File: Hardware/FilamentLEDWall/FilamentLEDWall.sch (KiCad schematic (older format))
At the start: 24 parts, among them J1 TopLeftConnector, J2 BottomLeftConnector, J3 BottomRightConnector, J4 TopRightConnector, U3 JXI5020GF

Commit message: Updated LED Board to v0.2
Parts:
- J1, J2, J3, J4: footprint Connector_PinHeader_2.54mm:PinHeader_2x04_P2.54mm_Vertical_SMD -> Connector_PinSocket_2.54mm:PinSocket_2x04_P2.54mm_Vertical_SMD
- U3: footprint Silicon-Standard:SSOP24 -> Sensor_Current:Allegro_QSOP-24_3.9x8.7mm_P0.635mm
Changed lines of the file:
@@
 F 0 "U3" H 8175 3515 50  0000 C CNN
 F 1 "JXI5020GF" H 8175 3424 50  0000 C CNN
-F 2 "Silicon-Standard:SSOP24" H 8500 3400 50  0001 C CNN
+F 2 "Sensor_Current:Allegro_QSOP-24_3.9x8.7mm_P0.635mm" H 8500 3400 50  0001 C CNN
 F 3 "" H 8500 3400 50  0001 C CNN
 	1    8200 2500
@@
 F 0 "J1" H 2900 6167 50  0000 C CNN
 F 1 "TopLeftConnector" H 2900 6076 50  0000 C CNN
-F 2 "Connector_PinHeader_2.54mm:PinHeader_2x04_P2.54mm_Vertical_SMD" H 2850 5850 50  0001 C CNN
+F 2 "Connector_PinSocket_2.54mm:PinSocket_2x04_P2.54mm_Vertical_SMD" H 2850 5850 50  0001 C CNN
 F 3 "~" H 2850 5850 50  0001 C CNN
 	1    2850 5850
@@
 F 0 "J2" H 2900 7167 50  0000 C CNN
 F 1 "BottomLeftConnector" H 2900 7076 50  0000 C CNN
-F 2 "Connector_PinHeader_2.54mm:PinHeader_2x04_P2.54mm_Vertical_SMD" H 2850 6850 50  0001 C CNN
+F 2 "Connector_PinSocket_2.54mm:PinSocket_2x04_P2.54mm_Vertical_SMD" H 2850 6850 50  0001 C CNN
 F 3 "~" H 2850 6850 50  0001 C CNN
 	1    2850 6850
@@
 F 0 "J4" H 4200 6167 50  0000 C CNN
 F 1 "TopRightConnector" H 4200 6076 50  0000 C CNN
-F 2 "Connector_PinHeader_2.54mm:PinHeader_2x04_P2.54mm_Vertical_SMD" H 4150 5850 50  0001 C CNN
+F 2 "Connector_PinSocket_2.54mm:PinSocket_2x04_P2.54mm_Vertical_SMD" H 4150 5850 50  0001 C CNN
 F 3 "~" H 4150 5850 50  0001 C CNN
 	1    4150 5850
@@
 F 0 "J3" H 4200 7167 50  0000 C CNN
 F 1 "BottomRightConnector" H 4200 7076 50  0000 C CNN
-F 2 "Connector_PinHeader_2.54mm:PinHeader_2x04_P2.54mm_Vertical_SMD" H 4150 6850 50  0001 C CNN
+F 2 "Connector_PinSocket_2.54mm:PinSocket_2x04_P2.54mm_Vertical_SMD" H 4150 6850 50  0001 C CNN
 F 3 "~" H 4150 6850 50  0001 C CNN
 	1    4150 6850

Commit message: updated wall cell and connector
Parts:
- U3: symbol CaoRX_Lib:JXI5020GF -> FilamentLEDWall-rescue:JXI5020GF-CaoRX_Lib
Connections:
- net 5V_LED: now also J1.1 (Pin_1), J2.1 (Pin_1), J3.1 (Pin_1), J4.1 (Pin_1); no longer J1.2 (Pin_2), J2.2 (Pin_2), J3.2 (Pin_2), J4.2 (Pin_2)
- net GND: now also J1.2 (Pin_2), J1.7 (Pin_7), J2.2 (Pin_2), J2.7 (Pin_7), J3.2 (Pin_2), J3.7 (Pin_7), J4.2 (Pin_2), J4.7 (Pin_7); no longer J1.1 (Pin_1), J1.8 (Pin_8), J2.1 (Pin_1), J2.8 (Pin_8), J3.1 (Pin_1), J3.8 (Pin_8), J4.1 (Pin_1), J4.8 (Pin_8)
- net LED_CLK: now also J1.4 (Pin_4), J2.4 (Pin_4), J3.4 (Pin_4), J4.4 (Pin_4); no longer J1.3 (Pin_3), J2.3 (Pin_3), J3.3 (Pin_3), J4.3 (Pin_3)
- net LED_LE: now also J1.6 (Pin_6), J2.6 (Pin_6), J3.6 (Pin_6), J4.6 (Pin_6); no longer J1.5 (Pin_5), J2.5 (Pin_5), J3.5 (Pin_5), J4.5 (Pin_5)
- net LED_OE: now also J1.8 (Pin_8), J2.8 (Pin_8), J3.8 (Pin_8), J4.8 (Pin_8); no longer J1.7 (Pin_7), J2.7 (Pin_7), J3.7 (Pin_7), J4.7 (Pin_7)
- net LED_SDI: now also J2.3 (Pin_3), J4.3 (Pin_3); no longer J2.4 (Pin_4), J4.4 (Pin_4)
- net LED_SDO: now also J1.5 (Pin_5), J3.5 (Pin_5); no longer J1.6 (Pin_6), J3.6 (Pin_6)

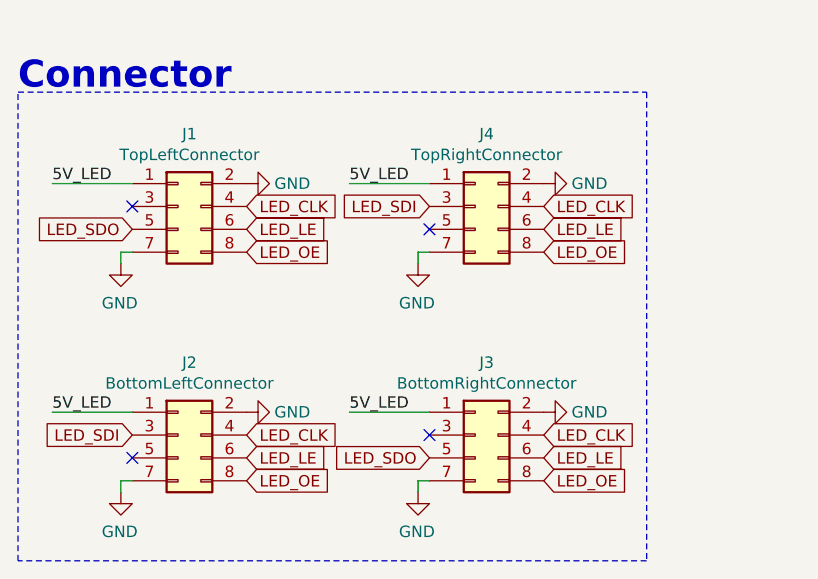
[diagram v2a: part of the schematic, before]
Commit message: merged all
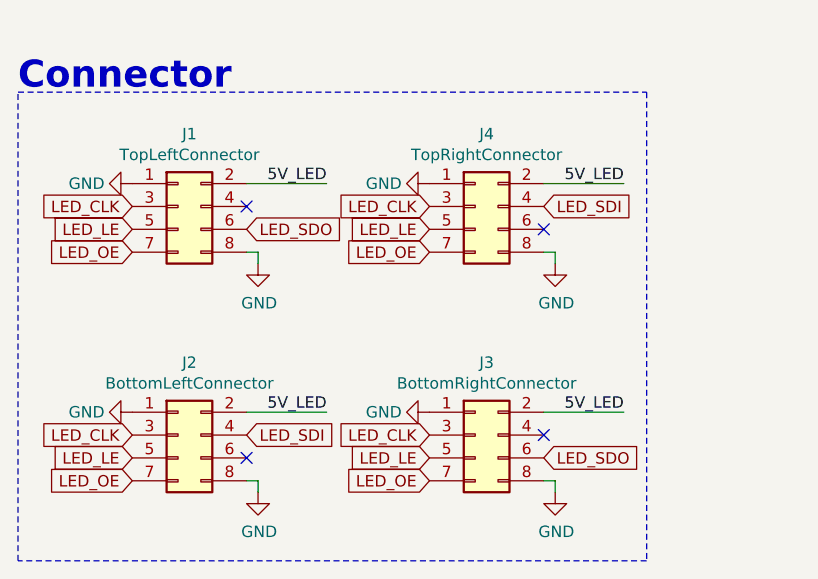
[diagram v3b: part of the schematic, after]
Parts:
- J1, J2, J3, J4: footprint Connector_PinSocket_2.54mm:PinSocket_2x04_P2.54mm_Vertical_SMD -> Connector_PinHeader_2.54mm:PinHeader_2x04_P2.54mm_Vertical_SMD
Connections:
- net 5V_LED: now also J1.2 (Pin_2), J2.2 (Pin_2), J3.2 (Pin_2), J4.2 (Pin_2); no longer J1.1 (Pin_1), J2.1 (Pin_1), J3.1 (Pin_1), J4.1 (Pin_1)
- net GND: now also J1.1 (Pin_1), J1.8 (Pin_8), J2.1 (Pin_1), J2.8 (Pin_8), J3.1 (Pin_1), J3.8 (Pin_8), J4.1 (Pin_1), J4.8 (Pin_8); no longer J1.2 (Pin_2), J1.7 (Pin_7), J2.2 (Pin_2), J2.7 (Pin_7), J3.2 (Pin_2), J3.7 (Pin_7), J4.2 (Pin_2), J4.7 (Pin_7)
- net LED_CLK: now also J1.3 (Pin_3), J2.3 (Pin_3), J3.3 (Pin_3), J4.3 (Pin_3); no longer J1.4 (Pin_4), J2.4 (Pin_4), J3.4 (Pin_4), J4.4 (Pin_4)
- net LED_LE: now also J1.5 (Pin_5), J2.5 (Pin_5), J3.5 (Pin_5), J4.5 (Pin_5); no longer J1.6 (Pin_6), J2.6 (Pin_6), J3.6 (Pin_6), J4.6 (Pin_6)
- net LED_OE: now also J1.7 (Pin_7), J2.7 (Pin_7), J3.7 (Pin_7), J4.7 (Pin_7); no longer J1.8 (Pin_8), J2.8 (Pin_8), J3.8 (Pin_8), J4.8 (Pin_8)
- net LED_SDI: now also J2.4 (Pin_4), J4.4 (Pin_4); no longer J2.3 (Pin_3), J4.3 (Pin_3)
- net LED_SDO: now also J1.6 (Pin_6), J3.6 (Pin_6); no longer J1.5 (Pin_5), J3.5 (Pin_5)
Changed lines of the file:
@@
 L power:GND #PWR0101
 U 1 1 6052D361
-P 2600 6100
-F 0 "#PWR0101" H 2600 5850 50  0001 C CNN
-F 1 "GND" H 2605 5927 50  0000 C CNN
-F 2 "" H 2600 6100 50  0001 C CNN
-F 3 "" H 2600 6100 50  0001 C CNN
-	1    2600 6100
-	-1   0    0    -1
-$EndComp
-Wire Wire Line
-	2650 6050 2600 6050
-Wire Wire Line
-	2600 6050 2600 6100
-Text Label 2300 5750 0    50   ~ 0
+P 3200 6100
+F 0 "#PWR0101" H 3200 5850 50  0001 C CNN
+F 1 "GND" H 3205 5927 50  0000 C CNN
+F 2 "" H 3200 6100 50  0001 C CNN
+F 3 "" H 3200 6100 50  0001 C CNN
+	1    3200 6100
+	1    0    0    -1
+$EndComp
+Wire Wire Line
+	3150 6050 3200 6050
+Wire Wire Line
+	3200 6050 3200 6100
+Text Label 3500 5750 2    50   ~ 0
 5V_LED
 Wire Notes Line
@@
 Connector
 Wire Wire Line
-	2650 5750 2300 5750
-Text GLabel 2650 5950 0    50   Input ~ 0
+	3150 5750 3500 5750
+Text GLabel 3150 5950 2    50   Input ~ 0
 LED_SDO
 Wire Wire Line
@@
 L power:GND #PWR0103
 U 1 1 60688380
-P 2600 7100
-F 0 "#PWR0103" H 2600 6850 50  0001 C CNN
-F 1 "GND" H 2605 6927 50  0000 C CNN
-F 2 "" H 2600 7100 50  0001 C CNN
-F 3 "" H 2600 7100 50  0001 C CNN
-	1    2600 7100
-	-1   0    0    -1
-$EndComp
-Wire Wire Line
-	2650 7050 2600 7050
-Wire Wire Line
-	2600 7050 2600 7100
-Text Label 2300 6750 0    50   ~ 0
-5V_LED
+P 3200 7100
+F 0 "#PWR0103" H 3200 6850 50  0001 C CNN
+F 1 "GND" H 3205 6927 50  0000 C CNN
+F 2 "" H 3200 7100 50  0001 C CNN
+F 3 "" H 3200 7100 50  0001 C CNN
+	1    3200 7100
+	1    0    0    -1
+$EndComp
+Wire Wire Line
+	3150 7050 3200 7050
+Wire Wire Line
+	3200 7050 3200 7100
+Text Label 3500 6750 2    50   ~ 0
+5V_LED
+Text GLabel 3150 6850 2    50   Input ~ 0
+LED_SDI
 Text GLabel 2650 6850 0    50   Input ~ 0
-LED_SDI
-Text GLabel 3150 6850 2    50   Input ~ 0
-LED_CLK
-Text GLabel 3150 6950 2    50   Input ~ 0
-LED_LE
-Text GLabel 3150 7050 2    50   Input ~ 0
-LED_OE
-Wire Wire Line
-	2650 6750 2300 6750
+LED_CLK
+Text GLabel 2650 6950 0    50   Input ~ 0
+LED_LE
+Text GLabel 2650 7050 0    50   Input ~ 0
+LED_OE
+Wire Wire Line
+	3150 6750 3500 6750
 $Comp
 L power:GND #PWR0104
 U 1 1 6068838F
-P 3150 6750
-F 0 "#PWR0104" H 3150 6500 50  0001 C CNN
-F 1 "GND" V 3150 6550 50  0000 C CNN
-F 2 "" H 3150 6750 50  0001 C CNN
-F 3 "" H 3150 6750 50  0001 C CNN
-	1    3150 6750
-	0    -1   1    0
+P 2650 6750
+F 0 "#PWR0104" H 2650 6500 50  0001 C CNN
+F 1 "GND" V 2650 6550 50  0000 C CNN
+F 2 "" H 2650 6750 50  0001 C CNN
+F 3 "" H 2650 6750 50  0001 C CNN
+	1    2650 6750
+	0    1    1    0
 $EndComp
 $Comp
@@
 F 0 "J2" H 2900 7167 50  0000 C CNN
 F 1 "BottomLeftConnector" H 2900 7076 50  0000 C CNN
-F 2 "Connector_PinSocket_2.54mm:PinSocket_2x04_P2.54mm_Vertical_SMD" H 2850 6850 50  0001 C CNN
+F 2 "Connector_PinHeader_2.54mm:PinHeader_2x04_P2.54mm_Vertical_SMD" H 2850 6850 50  0001 C CNN
 F 3 "~" H 2850 6850 50  0001 C CNN
 	1    2850 6850
 	1    0    0    -1
 $EndComp
-$Comp
-L power:GND #PWR0105
-U 1 1 6068AA6C
-P 3900 6100
-F 0 "#PWR0105" H 3900 5850 50  0001 C CNN
-F 1 "GND" H 3905 5927 50  0000 C CNN
-F 2 "" H 3900 6100 50  0001 C CNN
-F 3 "" H 3900 6100 50  0001 C CNN
-	1    3900 6100
-	-1   0    0    -1
-$EndComp
-Wire Wire Line
-	3950 6050 3900 6050
-Wire Wire Line
-	3900 6050 3900 6100
-Text Label 3600 5750 0    50   ~ 0
-5V_LED
 Text GLabel 3950 5850 0    50   Input ~ 0
-LED_SDI
-Text GLabel 4450 5850 2    50   Input ~ 0
-LED_CLK
-Text GLabel 4450 5950 2    50   Input ~ 0
-LED_LE
-Text GLabel 4450 6050 2    50   Input ~ 0
-LED_OE
-Wire Wire Line
-	3950 5750 3600 5750
+LED_CLK
+Text GLabel 3950 5950 0    50   Input ~ 0
+LED_LE
+Text GLabel 3950 6050 0    50   Input ~ 0
+LED_OE
 $Comp
 L power:GND #PWR0106
 U 1 1 6068AA7B
-P 4450 5750
-F 0 "#PWR0106" H 4450 5500 50  0001 C CNN
-F 1 "GND" V 4450 5550 50  0000 C CNN
-F 2 "" H 4450 5750 50  0001 C CNN
-F 3 "" H 4450 5750 50  0001 C CNN
-	1    4450 5750
-	0    -1   1    0
-$EndComp
-$Comp
-L Connector_Generic:Conn_02x04_Odd_Even J4
-U 1 1 6068AA81
-P 4150 5850
-F 0 "J4" H 4200 6167 50  0000 C CNN
-F 1 "TopRightConnector" H 4200 6076 50  0000 C CNN
-F 2 "Connector_PinSocket_2.54mm:PinSocket_2x04_P2.54mm_Vertical_SMD" H 4150 5850 50  0001 C CNN
-F 3 "~" H 4150 5850 50  0001 C CNN
-	1    4150 5850
-	1    0    0    -1
+P 3950 5750
+F 0 "#PWR0106" H 3950 5500 50  0001 C CNN
+F 1 "GND" V 3950 5550 50  0000 C CNN
+F 2 "" H 3950 5750 50  0001 C CNN
+F 3 "" H 3950 5750 50  0001 C CNN
+	1    3950 5750
+	0    1    1    0
 $EndComp
 $Comp
 L power:GND #PWR0107
 U 1 1 6068BAA0
-P 3900 7100
-F 0 "#PWR0107" H 3900 6850 50  0001 C CNN
-F 1 "GND" H 3905 6927 50  0000 C CNN
-F 2 "" H 3900 7100 50  0001 C CNN
-F 3 "" H 3900 7100 50  0001 C CNN
-	1    3900 7100
-	-1   0    0    -1
-$EndComp
-Wire Wire Line
-	3950 7050 3900 7050
-Wire Wire Line
-	3900 7050 3900 7100
-Text Label 3600 6750 0    50   ~ 0
-5V_LED
-Text GLabel 4450 6850 2    50   Input ~ 0
-LED_CLK
+P 4500 7100
+F 0 "#PWR0107" H 4500 6850 50  0001 C CNN
+F 1 "GND" H 4505 6927 50  0000 C CNN
+F 2 "" H 4500 7100 50  0001 C CNN
+F 3 "" H 4500 7100 50  0001 C CNN
+	1    4500 7100
+	1    0    0    -1
+$EndComp
+Wire Wire Line
+	4450 7050 4500 7050
+Wire Wire Line
+	4500 7050 4500 7100
+Text Label 4800 6750 2    50   ~ 0
+5V_LED
+Text GLabel 3950 6850 0    50   Input ~ 0
+LED_CLK
+Text GLabel 3950 6950 0    50   Input ~ 0
+LED_LE
+Text GLabel 3950 7050 0    50   Input ~ 0
+LED_OE
+Wire Wire Line
+	4450 6750 4800 6750
 Text GLabel 4450 6950 2    50   Input ~ 0
-LED_LE
-Text GLabel 4450 7050 2    50   Input ~ 0
-LED_OE
-Wire Wire Line
-	3950 6750 3600 6750
-Text GLabel 3950 6950 0    50   Input ~ 0
 LED_SDO
 $Comp
 L power:GND #PWR0108
 U 1 1 6068BAAF
-P 4450 6750
-F 0 "#PWR0108" H 4450 6500 50  0001 C CNN
-F 1 "GND" V 4450 6550 50  0000 C CNN
-F 2 "" H 4450 6750 50  0001 C CNN
-F 3 "" H 4450 6750 50  0001 C CNN
-	1    4450 6750
-	0    -1   1    0
+P 3950 6750
+F 0 "#PWR0108" H 3950 6500 50  0001 C CNN
+F 1 "GND" V 3950 6550 50  0000 C CNN
+F 2 "" H 3950 6750 50  0001 C CNN
+F 3 "" H 3950 6750 50  0001 C CNN
+	1    3950 6750
+	0    1    1    0
 $EndComp
 $Comp
@@
 F 0 "J3" H 4200 7167 50  0000 C CNN
 F 1 "BottomRightConnector" H 4200 7076 50  0000 C CNN
-F 2 "Connector_PinSocket_2.54mm:PinSocket_2x04_P2.54mm_Vertical_SMD" H 4150 6850 50  0001 C CNN
+F 2 "Connector_PinHeader_2.54mm:PinHeader_2x04_P2.54mm_Vertical_SMD" H 4150 6850 50  0001 C CNN
 F 3 "~" H 4150 6850 50  0001 C CNN
 	1    4150 6850
@@
 Text Notes 6800 4250 0    118  ~ 24
 Filter
-NoConn ~ 2650 5850
-NoConn ~ 3950 6850
-NoConn ~ 2650 6950
-NoConn ~ 3950 5950
+NoConn ~ 3150 5850
+NoConn ~ 4450 6850
+NoConn ~ 3150 6950
 $Comp
 L Connector_Generic:Conn_02x04_Odd_Even J1
@@
 F 0 "J1" H 2900 6167 50  0000 C CNN
 F 1 "TopLeftConnector" H 2900 6076 50  0000 C CNN
-F 2 "Connector_PinSocket_2.54mm:PinSocket_2x04_P2.54mm_Vertical_SMD" H 2850 5850 50  0001 C CNN
+F 2 "Connector_PinHeader_2.54mm:PinHeader_2x04_P2.54mm_Vertical_SMD" H 2850 5850 50  0001 C CNN
 F 3 "~" H 2850 5850 50  0001 C CNN
 	1    2850 5850
 	1    0    0    -1
 $EndComp
+NoConn ~ 4450 5950
+$Comp
+L Connector_Generic:Conn_02x04_Odd_Even J4
+U 1 1 6068AA81
+P 4150 5850
+F 0 "J4" H 4200 6167 50  0000 C CNN
+F 1 "TopRightConnector" H 4200 6076 50  0000 C CNN
+F 2 "Connector_PinHeader_2.54mm:PinHeader_2x04_P2.54mm_Vertical_SMD" H 4150 5850 50  0001 C CNN
+F 3 "~" H 4150 5850 50  0001 C CNN
+	1    4150 5850
+	1    0    0    -1
+$EndComp
+Wire Wire Line
+	4450 5750 4800 5750
+Text GLabel 4450 5850 2    50   Input ~ 0
+LED_SDI
+Text Label 4800 5750 2    50   ~ 0
+5V_LED
+Wire Wire Line
+	4500 6050 4500 6100
+Wire Wire Line
+	4450 6050 4500 6050
+$Comp
+L power:GND #PWR0105
+U 1 1 6068AA6C
+P 4500 6100
+F 0 "#PWR0105" H 4500 5850 50  0001 C CNN
+F 1 "GND" H 4505 5927 50  0000 C CNN
+F 2 "" H 4500 6100 50  0001 C CNN
+F 3 "" H 4500 6100 50  0001 C CNN
+	1    4500 6100
+	1    0    0    -1
+$EndComp
+Text GLabel 2650 5850 0    50   Input ~ 0
+LED_CLK
+Text GLabel 2650 5950 0    50   Input ~ 0
+LED_LE
+Text GLabel 2650 6050 0    50   Input ~ 0
+LED_OE
 $Comp
 L power:GND #PWR0102
 U 1 1 6063342B
-P 3150 5750
-F 0 "#PWR0102" H 3150 5500 50  0001 C CNN
-F 1 "GND" V 3150 5550 50  0000 C CNN
-F 2 "" H 3150 5750 50  0001 C CNN
-F 3 "" H 3150 5750 50  0001 C CNN
-	1    3150 5750
-	0    -1   1    0
-$EndComp
-Text GLabel 3150 6050 2    50   Input ~ 0
-LED_OE
-Text GLabel 3150 5950 2    50   Input ~ 0
-LED_LE
-Text GLabel 3150 5850 2    50   Input ~ 0
-LED_CLK
+P 2650 5750
+F 0 "#PWR0102" H 2650 5500 50  0001 C CNN
+F 1 "GND" V 2650 5550 50  0000 C CNN
+F 2 "" H 2650 5750 50  0001 C CNN
+F 3 "" H 2650 5750 50  0001 C CNN
+	1    2650 5750
+	0    1    1    0
+$EndComp
 $EndSCHEMATC
